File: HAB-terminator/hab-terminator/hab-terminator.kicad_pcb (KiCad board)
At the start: 2 copper layers, 25 x 63.3 mm, 42 parts, among them J1 Battery, J2 Burn wire, J3 Actuator, J4 MSD-4-A, J5 Heater, Q1 DMN2053UVTQ-7, Q2 DMN2053UVTQ-7, Q3 AO3401A, Q4 AO3401A, SW2 SW_Push_EXT, U1 XIAO-ESP32-C3-SMD, U2 DRV8212P, U3 74LVC1G3157, U4 MS5607-02BA

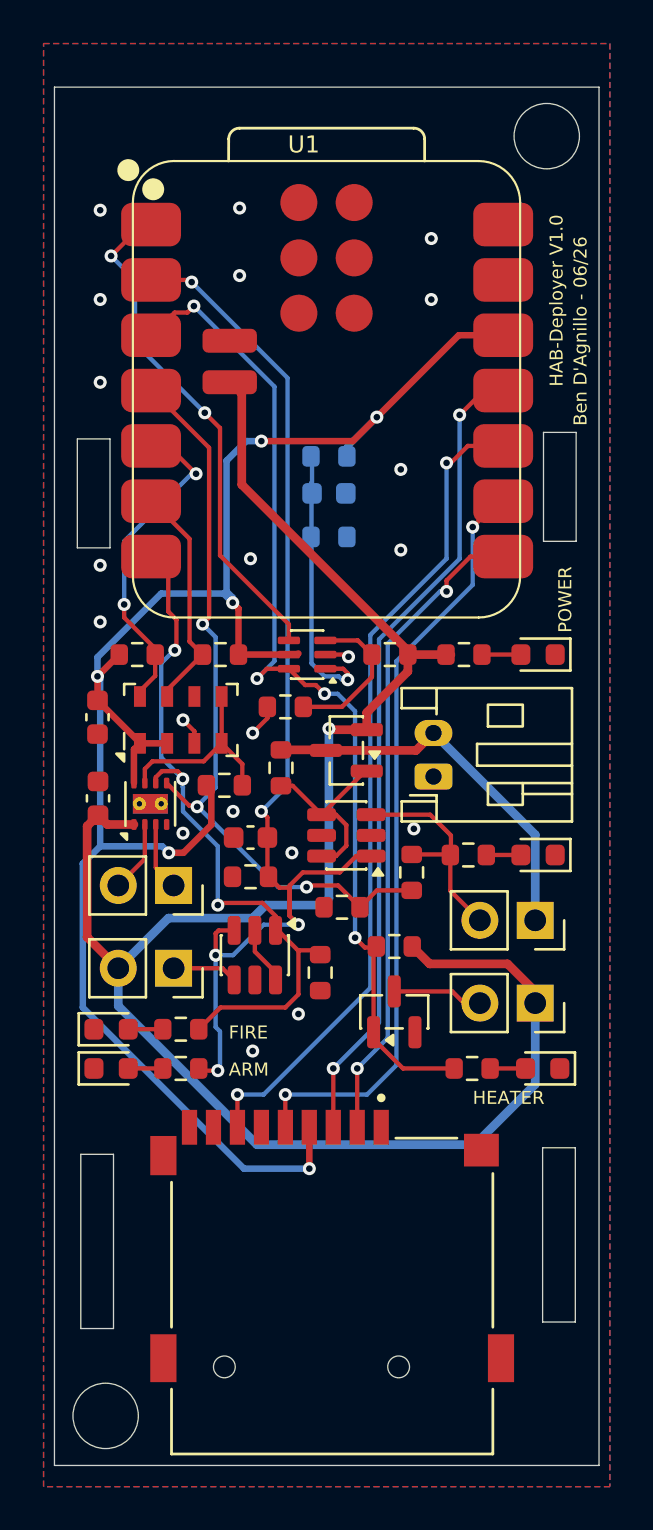
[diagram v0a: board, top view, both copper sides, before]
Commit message: updating terminator
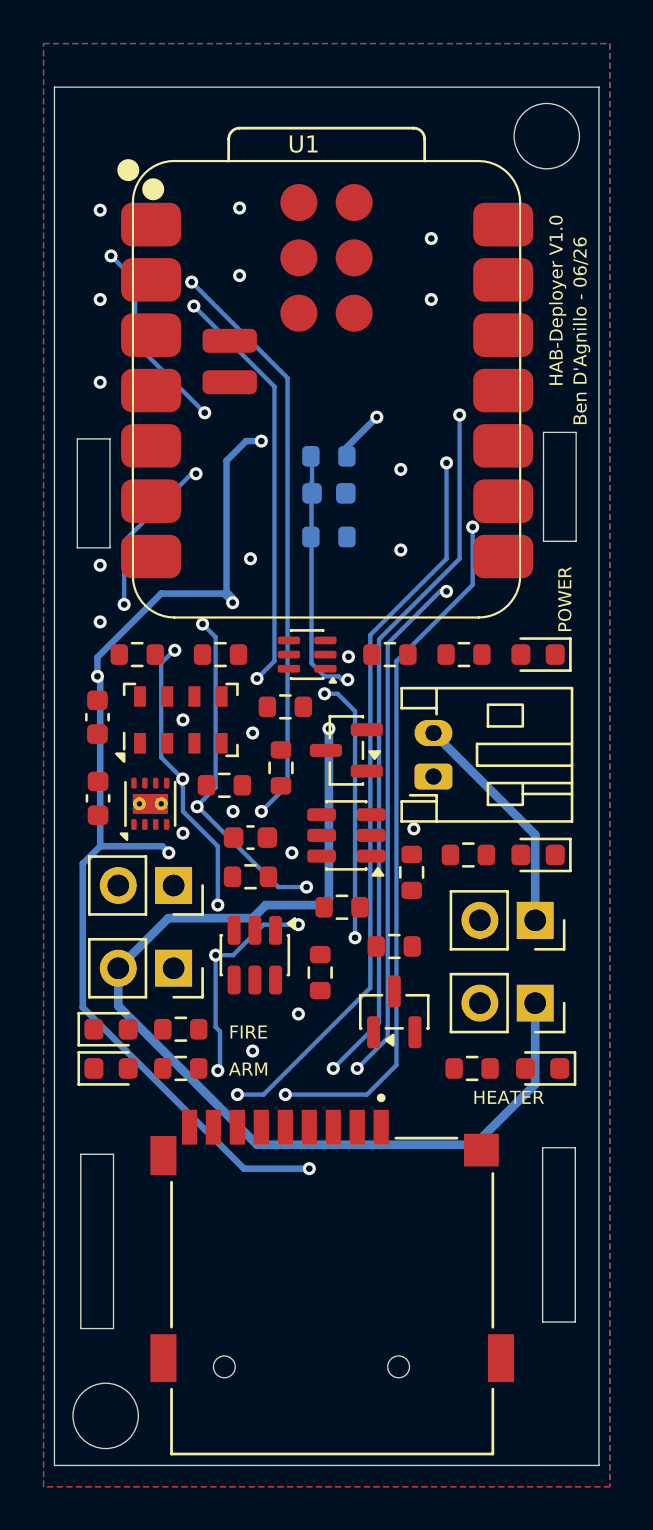
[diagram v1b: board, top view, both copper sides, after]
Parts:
- R14, R15: value 4.7k -> 10k
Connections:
- Q3 pad 2: +BATT -> /VBAT
- Q3 pad 3: /VBAT -> +BATT
- Q4 pad 2: GND -> Net-(J5-Pin_2)
- Q4 pad 3: Net-(J5-Pin_2) -> GND
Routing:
- net +BATT: track 87.7 -> 47.2 mm
- net +3V3: track 84.9 -> 51.8 mm
- net /BURN_EN/ACT_1: track 33.2 -> 13.0 mm
- net /SW_SNS/ACT_2: track 34.9 -> 15.5 mm
- net /BURN_ARM/PWR_HOLD: track 53.0 -> 36.4 mm
- net /HEATER_EN/A_MUX: track 47.1 -> 31.1 mm
- net /NTC/VBAT_SNS: track 23.5 -> 8.98 mm
- net /I2C_SDA: track 10.6 -> 0.00 mm
- net Net-(Q2B-G): track 10.3 -> 0.00 mm
- net /CSB/~{SLEEP}: track 9.33 -> 0.00 mm
- net Net-(Q2A-D): track 8.93 -> 0.00 mm
- net /I2C_SCL: track 15.1 -> 7.48 mm
- net /VBAT: track 17.9 -> 10.5 mm
- net Net-(R20-Pad2): track 7.15 -> 0.00 mm
- net /SD_CS: track 30.2 -> 23.8 mm
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- added copper zone on In1.Cu, net +3V3
- added copper zone on In2.Cu, net GND
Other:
- copper layers 2 -> 4
